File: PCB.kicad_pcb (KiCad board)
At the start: 2 copper layers, 29 parts, among them J1 Conn_01x03_Male, J2 Conn_01x04_Male, J3 Conn_02x03_Odd_Even, J4 Conn_01x03_Male, U1 L7805, U2 TMA1215D, U3 ATTINY2313-20PU, U4 DAC0808_DIP, U5 LM358, U6 DS18B20, U7 MAX485E, Y1 Crystal

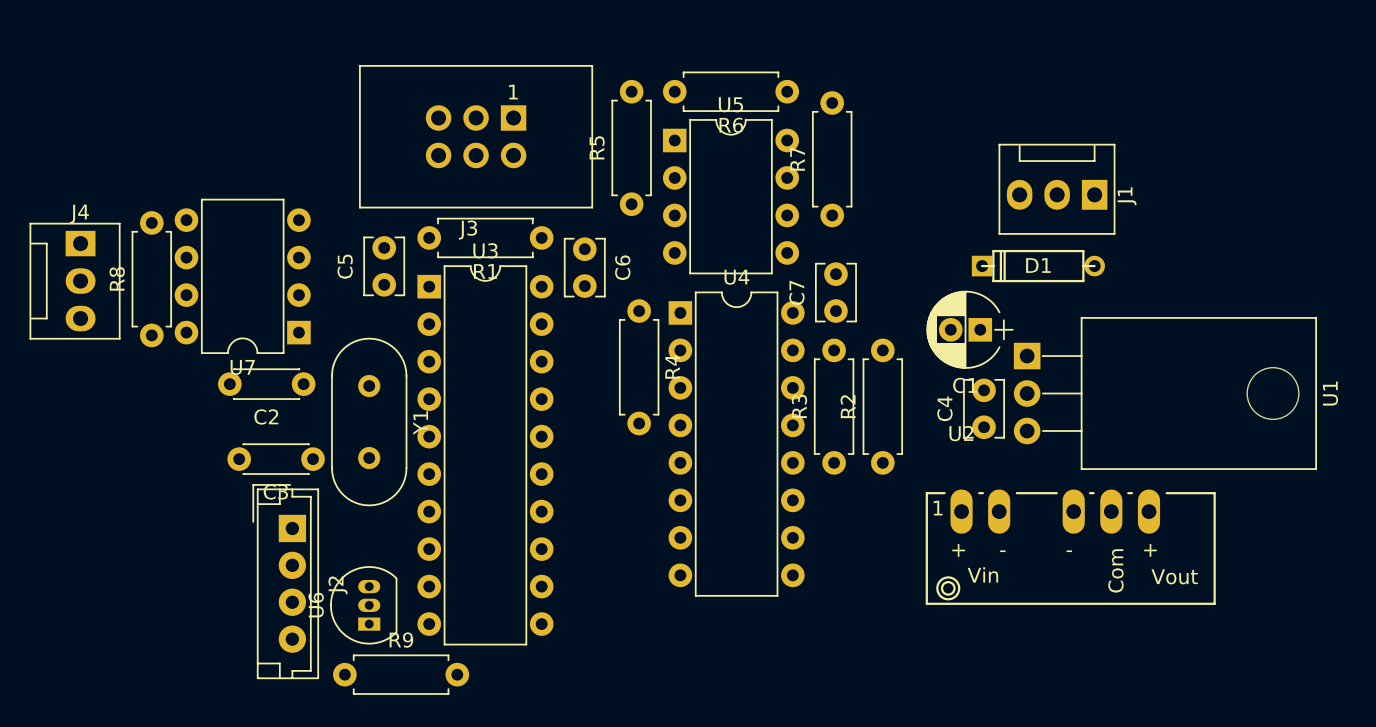
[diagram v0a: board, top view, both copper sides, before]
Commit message: PCB erstellt
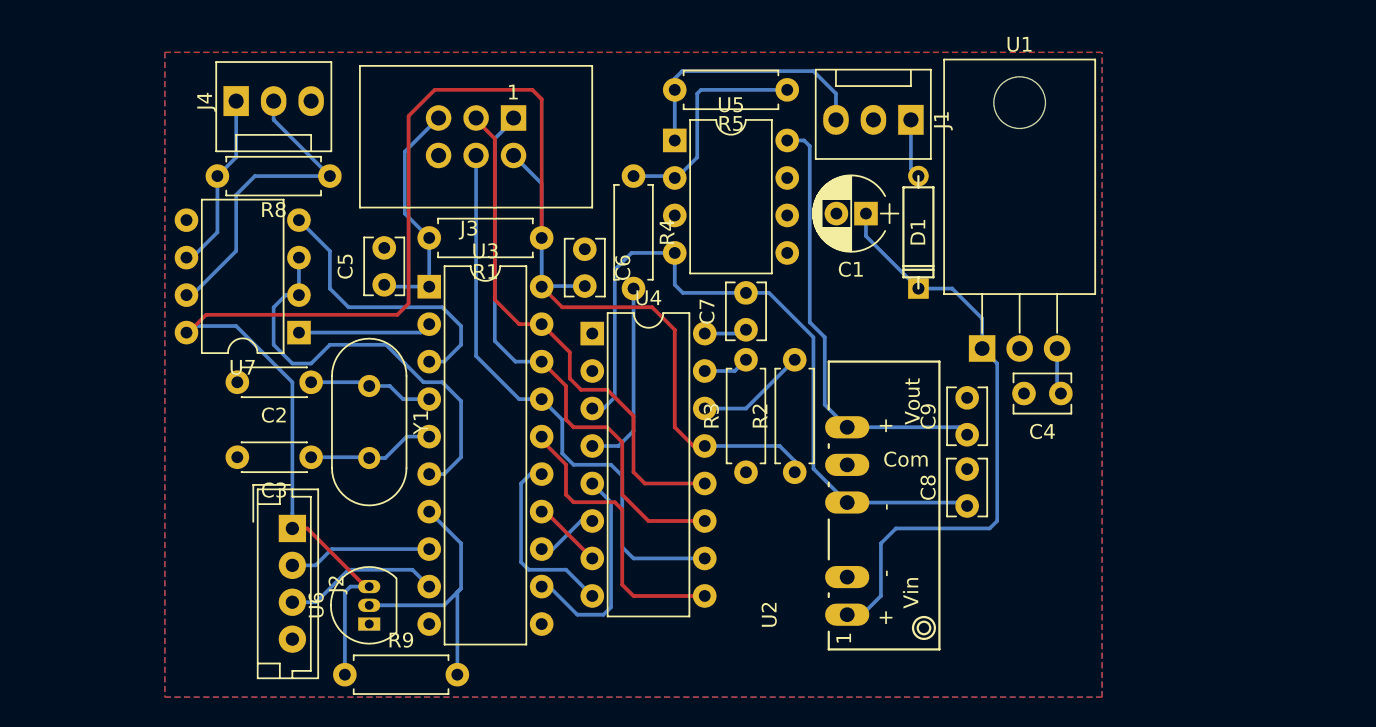
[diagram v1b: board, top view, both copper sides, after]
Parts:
- removed R6, R7: R, Resistors_THT:R_Axial_DIN0207_L6.3mm_D2.5mm_P7.62mm_Horizontal
- added C8: C, Capacitors_THT:C_Disc_D3.8mm_W2.6mm_P2.50mm, F.Cu at (148.6, 108.7)
- added C9: C, Capacitors_THT:C_Disc_D3.8mm_W2.6mm_P2.50mm, F.Cu at (148.6, 103.9)
- moved R8 16.2 mm to (105.4, 86.4), turned to 180 degrees
- moved J4 14.3 mm to (99.1, 81.3), turned to 90 degrees
- moved J1 13.4 mm to (144.8, 82.5)
- moved R5 13.1 mm to (136.4, 80.5), turned to 180 degrees
- moved C1 11.0 mm to (141.7, 88.9)
- moved U2 10.4 mm to (140.5, 116.1), turned to 90 degrees
- moved R4 9.15 mm to (126.0, 86.4)
- moved D1 8.44 mm to (145.3, 90.2), turned to 270 degrees
- moved C7 6.23 mm to (133.6, 96.8)
- moved U4 6.13 mm to (123.2, 97.0)
- moved R2 6.00 mm to (136.9, 106.4)
- moved R3 6.00 mm to (133.6, 106.4)
- moved C4 5.69 mm to (154.9, 101.1), turned to 180 degrees
- moved U1 3.09 mm to (149.6, 98.0), turned to 0 degrees
- moved C2 0.52 mm to (104.1, 100.3)
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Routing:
- net VCC: track 0.00 -> 120.3 mm
- net -15V: track 0.00 -> 48.4 mm
- net VDD: track 0.00 -> 40.7 mm
- net /MOSI: track 0.00 -> 38.9 mm
- net /MISO: track 0.00 -> 38.6 mm
- net /PB7: track 0.00 -> 35.5 mm
- net +15V: track 0.00 -> 30.1 mm
- net /DR: track 0.00 -> 28.9 mm
- net Net-(J4-Pad2): track 0.00 -> 21.9 mm
- net /PB4: track 0.00 -> 19.8 mm
- net /TXD: track 0.00 -> 19.3 mm
- net /OneWire: track 0.00 -> 18.7 mm
- net /AnalogOut: track 0.00 -> 17.7 mm
- net Net-(R4-Pad1): track 0.00 -> 16.3 mm
- net /RESET: track 0.00 -> 16.2 mm
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- added copper zone on B.Cu, net GND
- added copper zone on F.Cu, net GND
